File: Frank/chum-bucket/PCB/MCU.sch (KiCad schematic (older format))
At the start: 61 parts, among them J205 CAN_CONN, J206 SWD_DIAGS, SW201 B3U-1000P, SW202 LV_EN, SW203 SW_SPST, U215 STM32F042K6Tx, U216 TPS70933DRVT, Y201 32MHz

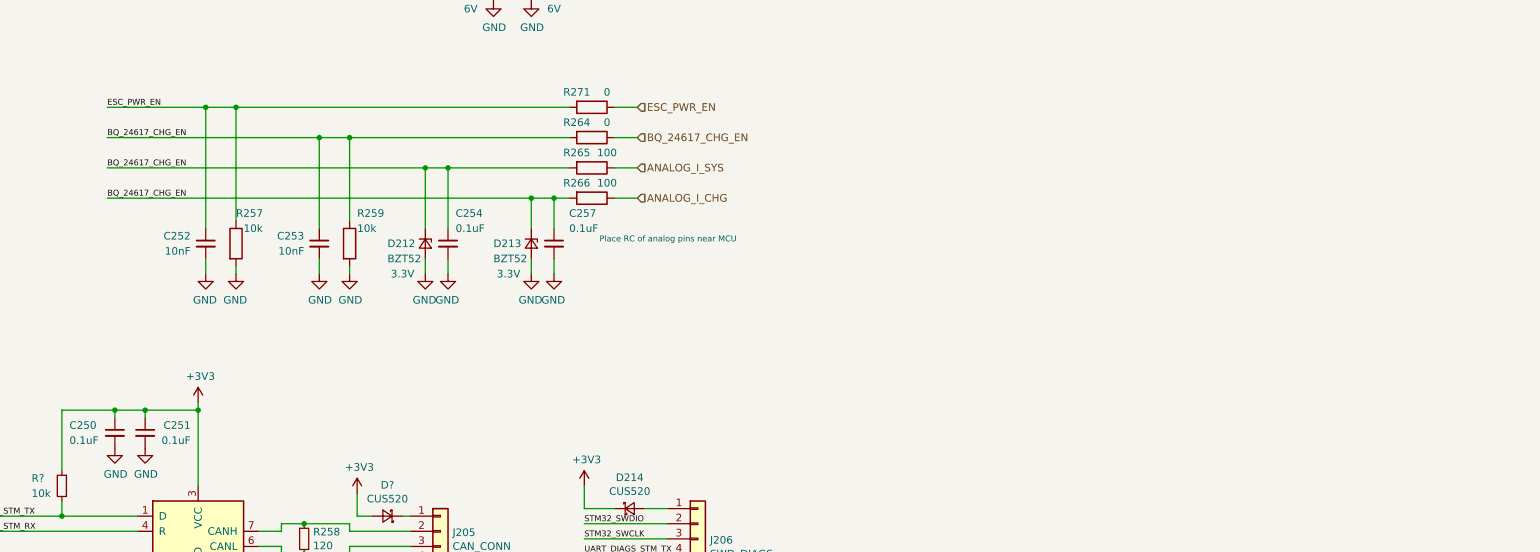
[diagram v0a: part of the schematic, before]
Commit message: more changes :)
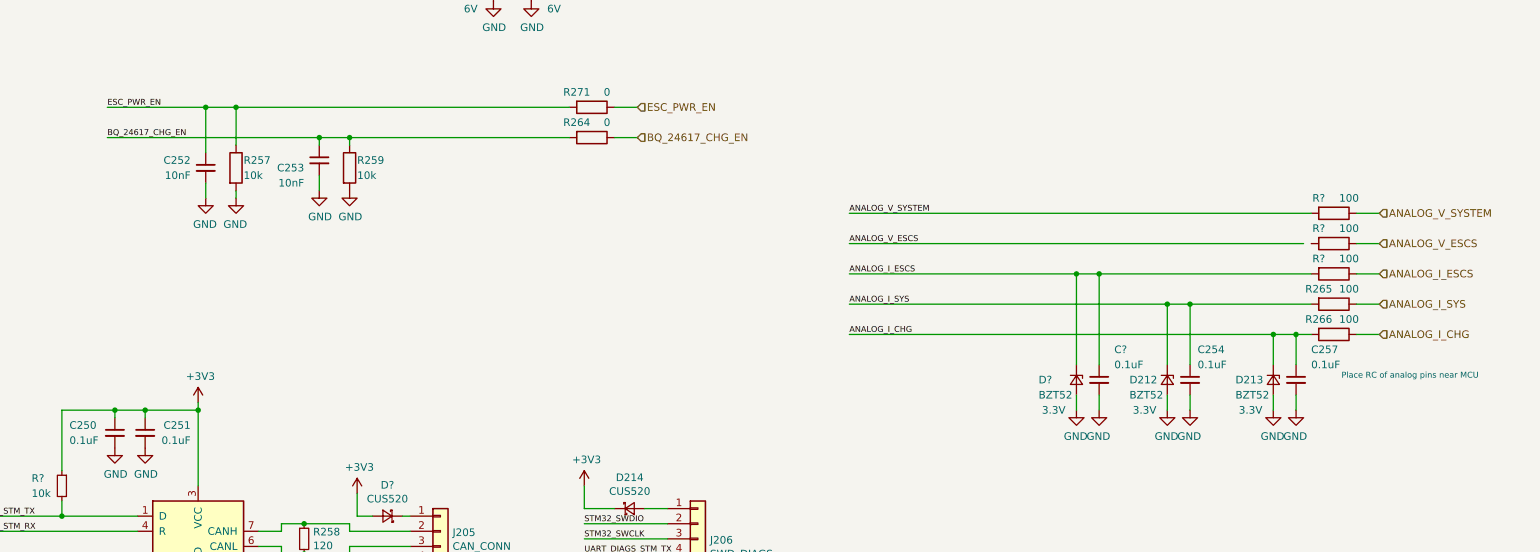
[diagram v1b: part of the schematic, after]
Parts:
- added C?: 0.1uF, Capacitor_SMD:C_0603_1608Metric, symbol Device:C_Small
- added D?: BZT52, Diode_SMD:D_SOD-123, symbol Device:D_Zener_Small
- added R? (x3): 100, Resistor_SMD:R_0603_1608Metric, symbol Device:R
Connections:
- net ANALOG_I_CHG: now also C257.1, D213.1 (K), R266.2
- net ANALOG_I_SYS: now also C254.1, D212.1 (K), R265.2
- net BQ_24617_CHG_EN: no longer C254.1, C257.1, D212.1 (K), D213.1 (K), R265.2, R266.2
- net GND: now also C?.2, D?.2 (A)
- new net ANALOG_I_ESCS: C?.1, D?.1 (K), R?.1, R?.2
- new net ANALOG_V_ESCS: R?.1
- new net ANALOG_V_SYSTEM: R?.1, R?.2
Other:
- moved on the sheet: C252, C253, C254, C257, D212, D213, R257, R259, R265, R266
